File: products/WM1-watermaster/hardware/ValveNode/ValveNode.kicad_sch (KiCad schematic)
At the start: 42 parts, among them J2 Conn_Coaxial_Small, J3 PWR_CONN, J5 Conn_01x05_Pin, U10 DRV8871DDA, U11 74HC595, U13 AMS1117-5.0, U2 74HC595, U4 DRV8871DDA, U5 ESP32 30 Pin CP2102 Developme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, U6 DRV8871DDA, U7 ISC-SX1262-B, U8 AP2112K-3.3, U9 DRV8871DDA

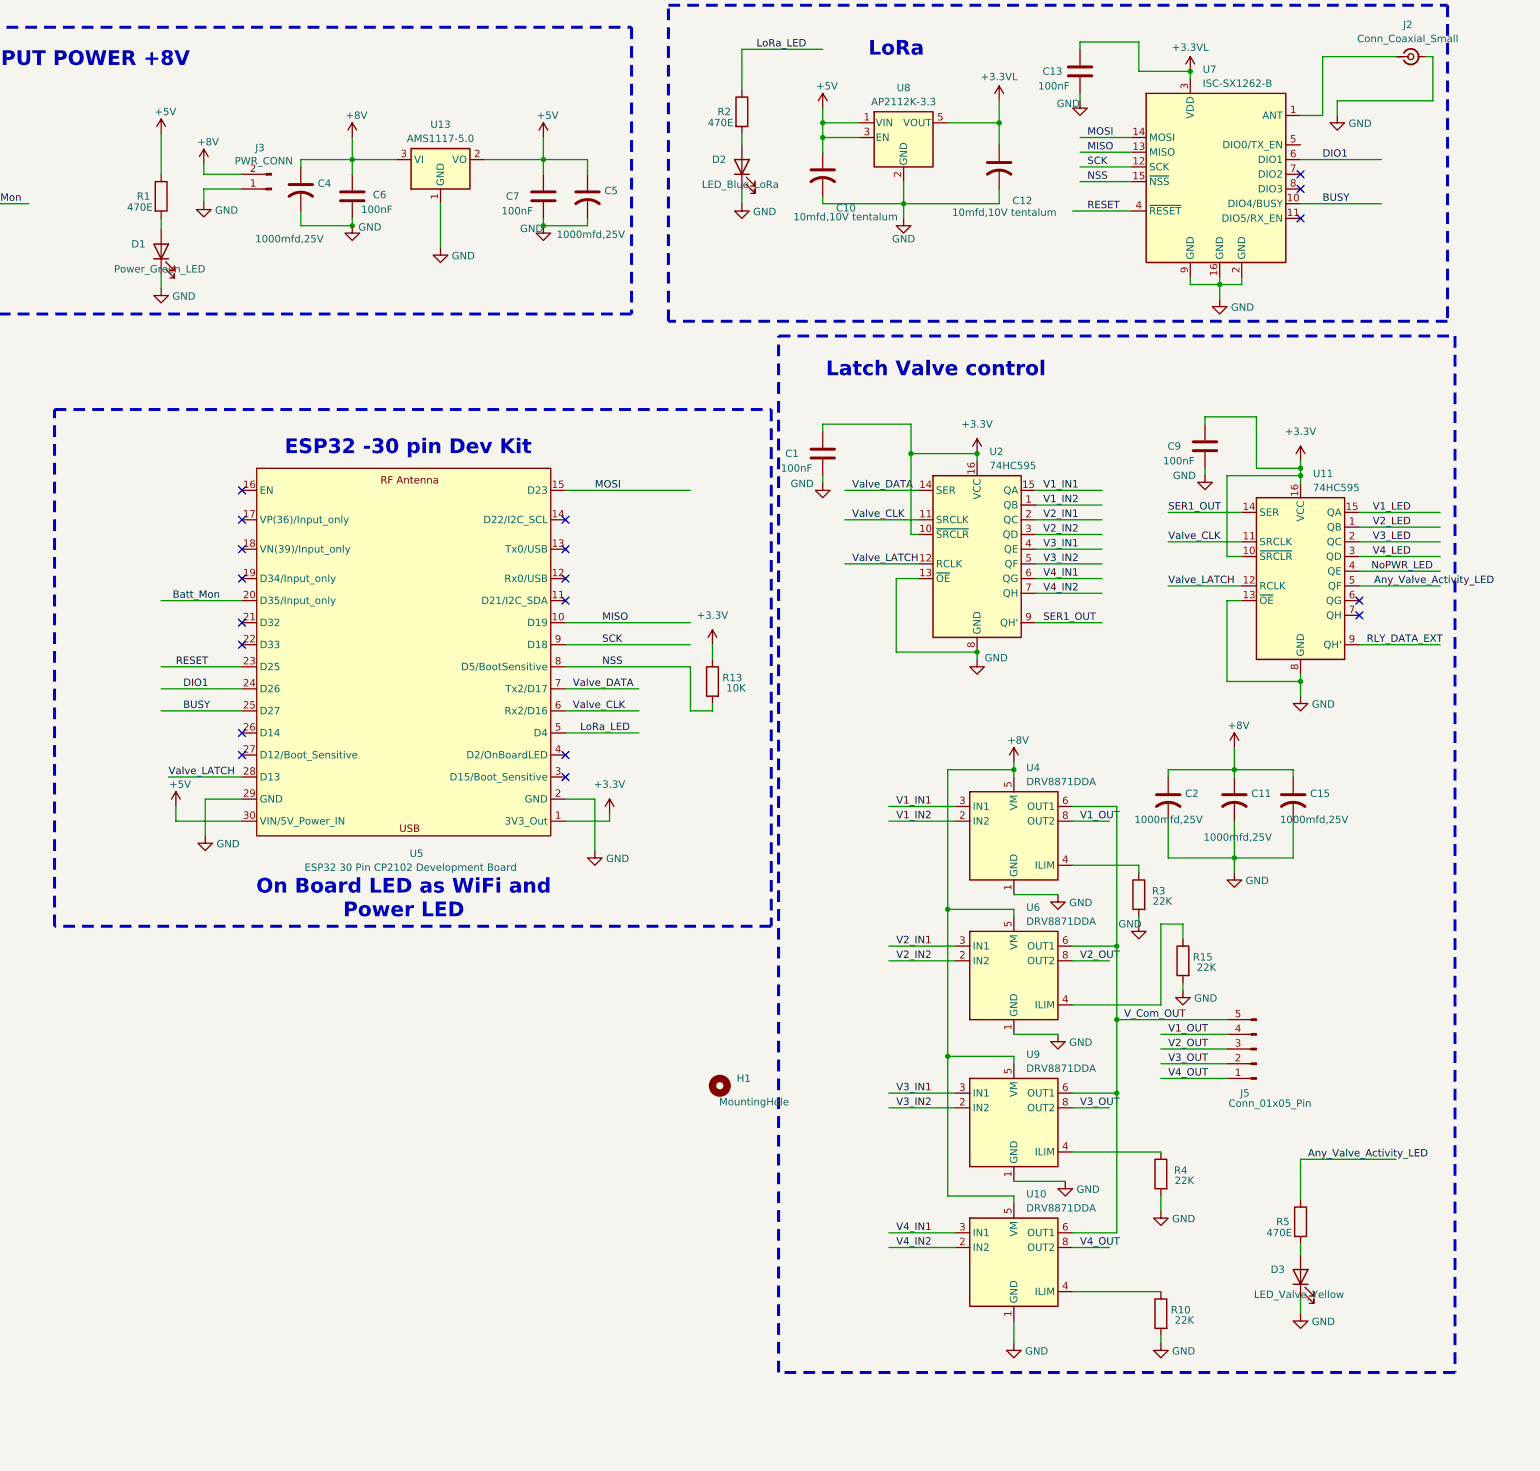
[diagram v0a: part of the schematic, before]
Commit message: updated Valve Node-V4
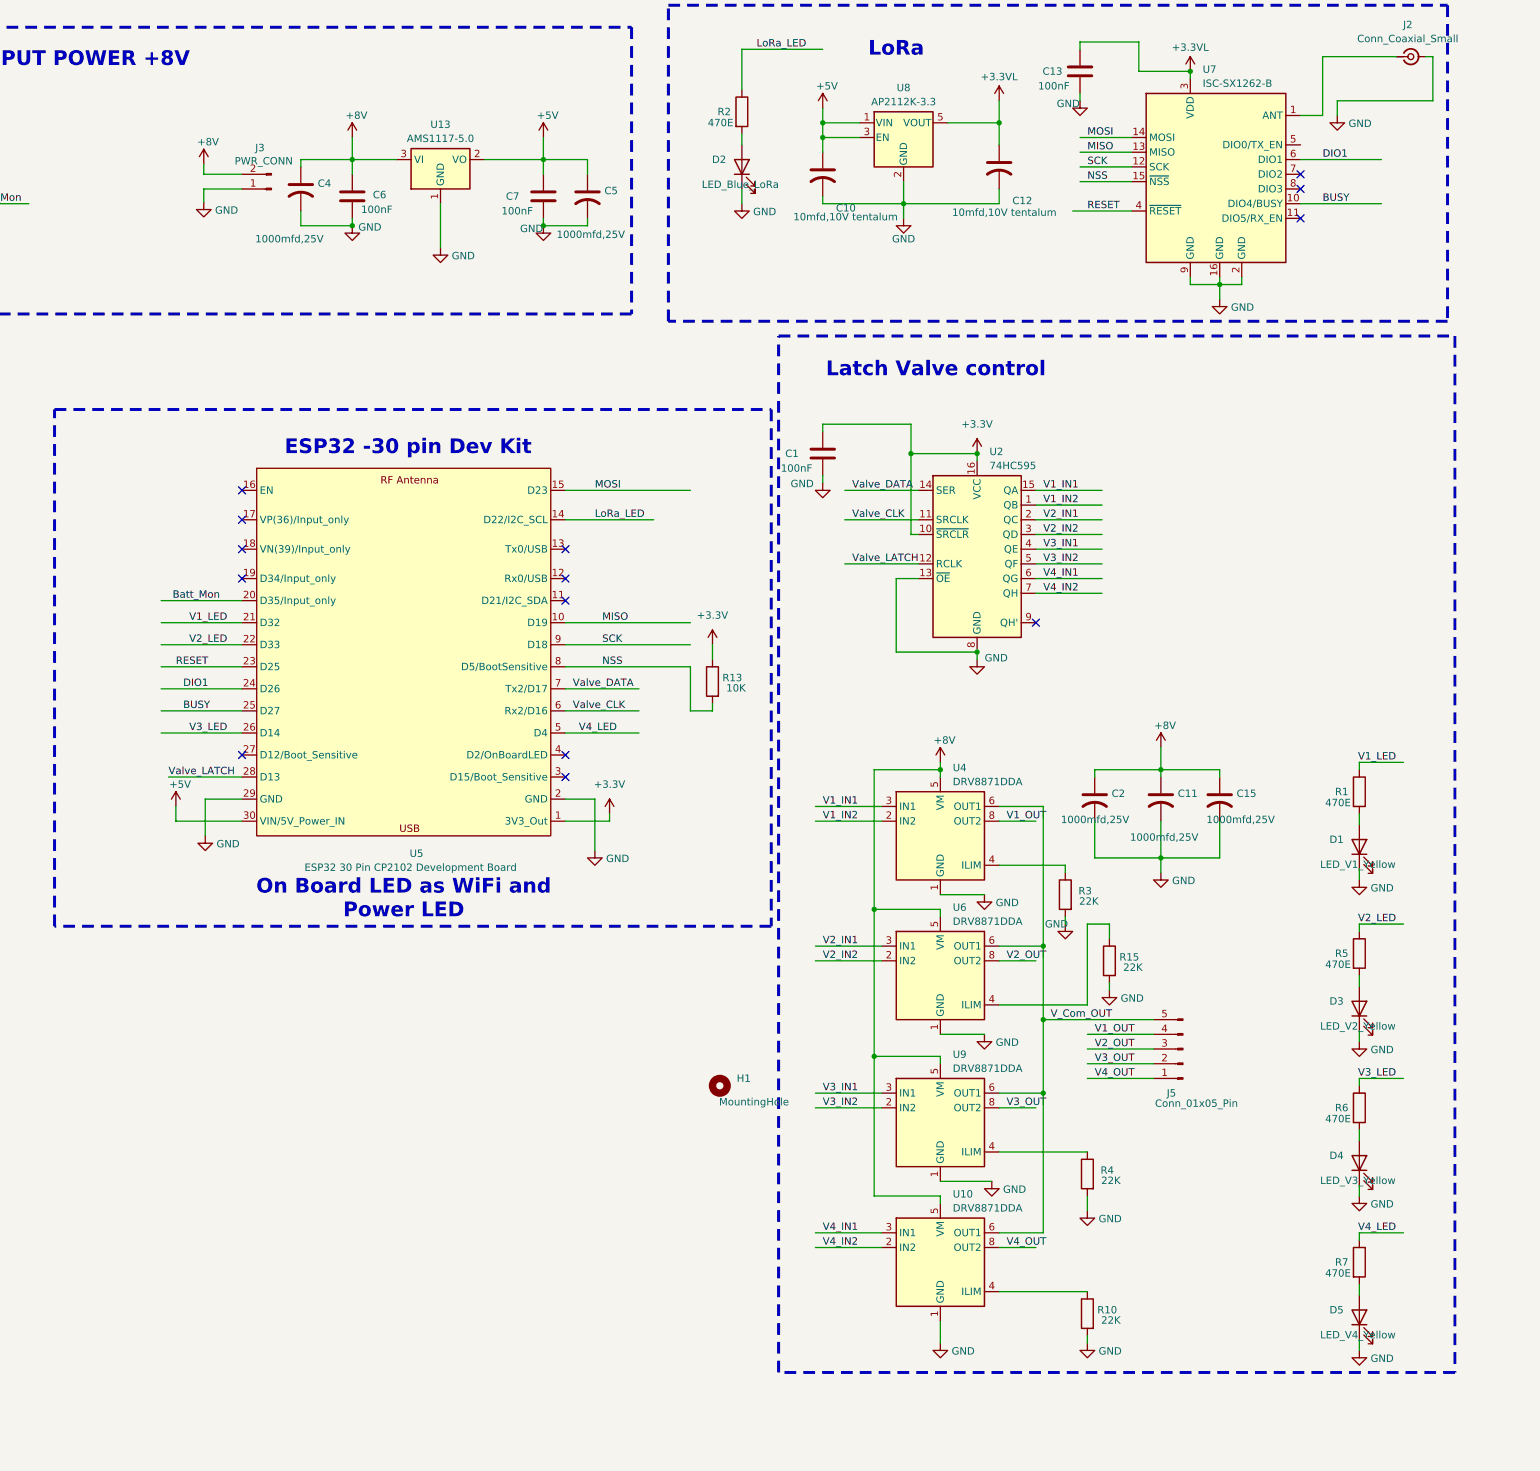
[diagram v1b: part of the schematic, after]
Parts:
- removed C9: 100nF, Capacitor_SMD:C_0805_2012Metric, symbol Device:C
- removed U11: 74HC595, Package_SO:SOIC-16_3.9x9.9mm_P1.27mm, symbol 74xx:74HC595
- added D4: LED_V3_Yellow, LED_0805_2012Metric_Pad1.15x1.40mm_HandSolder, symbol Device:LED
- added D5: LED_V4_Yellow, LED_0805_2012Metric_Pad1.15x1.40mm_HandSolder, symbol Device:LED
- added R6, R7: 470E, Resistor_SMD:R_0805_2012Metric, symbol Device:R
- D1: value Power_Green_LED -> LED_V1_Yellow; footprint LED_THT:LED_D3.0mm -> LED_0805_2012Metric_Pad1.15x1.40mm_HandSolder
- D2: footprint LED_THT:LED_D3.0mm -> LED_0805_2012Metric_Pad1.15x1.40mm_HandSolder
- D3: value LED_Valve_Yellow -> LED_V2_Yellow; footprint LED_THT:LED_D3.0mm -> LED_0805_2012Metric_Pad1.15x1.40mm_HandSolder
- J3: footprint PhoenixContact_MSTBA_2,5_2-G-5,08_1x02_P5.08mm_Horizontal -> Connector_Phoenix_MSTB:PhoenixContact_MSTBVA_2,5_2-G-5,08_1x02_P5.08mm_Vertical
- J5: footprint Connector_Phoenix_MSTB:PhoenixContact_MSTBA_2,5_5-G-5,08_1x05_P5.08mm_Horizontal -> Connector_Phoenix_MSTB:PhoenixContact_MSTBVA_2,5_5-G-5,08_1x05_P5.08mm_Vertical
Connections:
- net Any_Valve_Activity_LED is gone; now on net V2_LED: R5.1
- net +5V: no longer R1.1
- net GND: now also D4.1 (K), D5.1 (K)
- net LoRa_LED: now also U5.14 (D22/I2C_SCL); no longer U5.5 (D4)
- net V1_LED: now also R1.1, U5.21 (D32)
- net V2_LED: now also U5.22 (D33)
- net V3_LED: now also U5.26 (D14), R6.1
- net V4_LED: now also U5.5 (D4), R7.1
- net SER1_OUT: no longer names the net of U2.9 (QH')
- new net: D4.2 (A), R6.2
- new net: D5.2 (A), R7.2
- no-connect marks 19 -> 14
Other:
- moved on the sheet: C11, C15, C2, J5, R10, R15, R3, R4, U10, U4, U6, U9
